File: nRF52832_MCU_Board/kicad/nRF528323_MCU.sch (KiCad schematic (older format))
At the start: 34 parts, among them J6 DEBUG_CONNECTOR, J7 CONN_01X05, J8 MM8130-2600, X1 32MHz, X2 32.768kHz

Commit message: Update KiCad Project nRF52832_MCU_Board
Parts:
- J6: footprint Nordic_misc:Pin_Header_Straight_2x05_Pitch1.27mm_SMD -> Nordic_misc:ftsh-105-01-l-dv
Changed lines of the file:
@@
 F 0 "J6" H 7500 5200 50  0000 C CNN
 F 1 "DEBUG_CONNECTOR" H 7500 4600 50  0000 C CNN
-F 2 "Nordic_misc:Pin_Header_Straight_2x05_Pitch1.27mm_SMD" H 7500 3700 50  0001 C CNN
+F 2 "Nordic_misc:ftsh-105-01-l-dv" H 7500 3700 50  0001 C CNN
 F 3 "" H 7500 3700 50  0001 C CNN
 	1    7500 4900

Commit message: Update KiCAD Project nRF52832_MCU_Board
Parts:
- X1: footprint Crystals:Crystal_SMD_2016-4pin_2.0x1.6mm -> Nordic_nRF:Crystal_SMD_2016-4pin_2.0x1.6mm
- X2: footprint Crystals:Crystal_SMD_3215-2pin_3.2x1.5mm -> Nordic_nRF:Crystal_SMD_3215-2pin_3.2x1.5mm
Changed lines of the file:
@@
 $Descr USLetter 11000 8500
 encoding utf-8
-Sheet 2 4
+Sheet 4 4
 Title ""
 Date "2017-07-22"
@@
 F 0 "X2" V 2000 2950 50  0000 C CNN
 F 1 "32.768kHz" V 2150 3050 50  0000 C CNN
-F 2 "Crystals:Crystal_SMD_3215-2pin_3.2x1.5mm" H 2050 2800 50  0001 C CNN
+F 2 "Nordic_nRF:Crystal_SMD_3215-2pin_3.2x1.5mm" H 2050 2800 50  0001 C CNN
 F 3 "" H 2050 2800 50  0001 C CNN
 	1    2050 2800
@@
 F 0 "X1" V 8450 2500 50  0000 L CNN
 F 1 "32MHz" V 8550 2300 50  0000 L CNN
-F 2 "Crystals:Crystal_SMD_2016-4pin_2.0x1.6mm" H 8650 2700 50  0001 C CNN
+F 2 "Nordic_nRF:Crystal_SMD_2016-4pin_2.0x1.6mm" H 8650 2700 50  0001 C CNN
 F 3 "" H 8650 2700 50  0001 C CNN
 	1    8650 2700

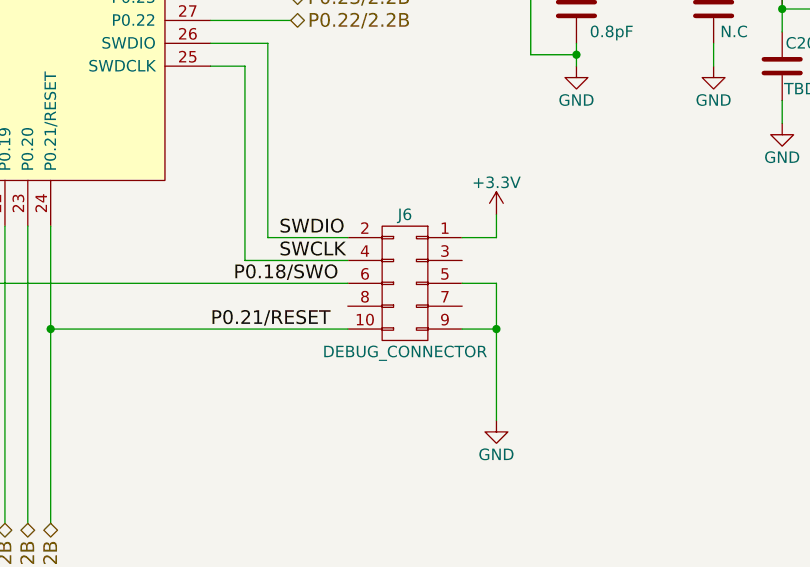
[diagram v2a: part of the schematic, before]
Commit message: Update KiCAD Project nRF52832_MCU_Board
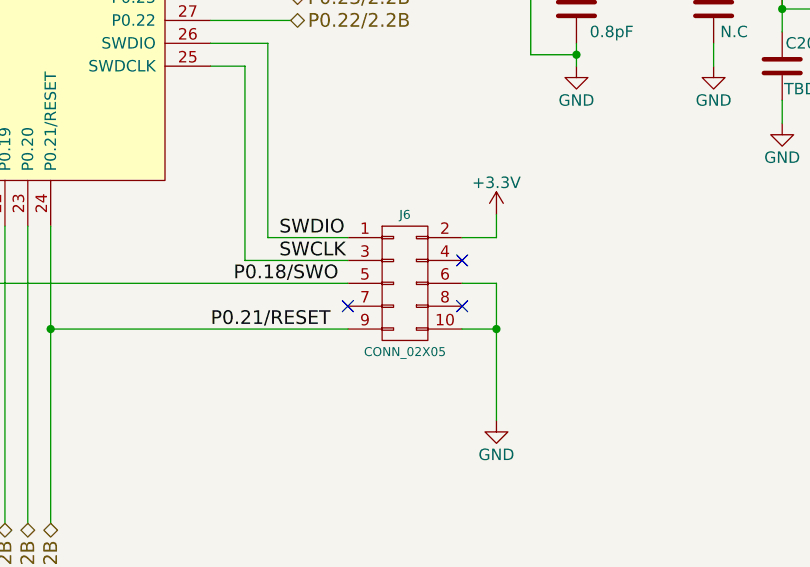
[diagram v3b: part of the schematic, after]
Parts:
- J6: value DEBUG_CONNECTOR -> CONN_02X05
- nRF1: footprint nRF52:UQFN-48-1EP_6x6mm_Pitch0.4mm -> Nordic_nRF:Nordic_nRF-QFN40P600X600X90-48_N
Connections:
- net +3V3: now also J6.2 (P2); no longer J6.1 (P1)
- net GND: now also J6.10 (P10), J6.6 (P6); no longer J6.5 (P5), J6.9 (P9)
- net P0.18/SWO/2.2B: now also J6.5 (P5); no longer J6.6 (P6)
- net P0.21/RESET/2.2B: now also J6.9 (P9); no longer J6.10 (P10)
- net SWCLK: now also J6.3 (P3); no longer J6.4 (P4)
- net SWDIO: now also J6.1 (P1); no longer J6.2 (P2)
- no-connect marks 3 -> 6
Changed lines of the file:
@@
 EESchema Schematic File Version 2
-LIBS:power
-LIBS:device
-LIBS:transistors
-LIBS:conn
-LIBS:linear
-LIBS:regul
+LIBS:nRF52832_MCU_Board-rescue
+LIBS:Nordic_misc
+LIBS:Nordic_nRF
+LIBS:74xgxx
 LIBS:74xx
-LIBS:cmos4000
-LIBS:adc-dac
-LIBS:memory
-LIBS:xilinx
-LIBS:microcontrollers
-LIBS:dsp
-LIBS:microchip
-LIBS:analog_switches
-LIBS:motorola
-LIBS:texas
-LIBS:intel
-LIBS:audio
-LIBS:interface
-LIBS:digital-audio
-LIBS:philips
-LIBS:display
-LIBS:cypress
-LIBS:siliconi
-LIBS:opto
-LIBS:atmel
-LIBS:contrib
-LIBS:valves
-LIBS:74xgxx
 LIBS:ac-dc
 LIBS:actel
+LIBS:adc-dac
 LIBS:allegro
 LIBS:Altera
 LIBS:analog_devices
+LIBS:analog_switches
+LIBS:atmel
+LIBS:audio
 LIBS:battery_management
 LIBS:bbd
@@
 LIBS:brooktre
 LIBS:cmos_ieee
+LIBS:cmos4000
+LIBS:conn
+LIBS:contrib
+LIBS:cypress
 LIBS:dc-dc
+LIBS:device
+LIBS:digital-audio
 LIBS:diode
+LIBS:display
+LIBS:dsp
 LIBS:elec-unifil
 LIBS:ESD_Protection
@@
 LIBS:graphic
 LIBS:hc11
+LIBS:intel
+LIBS:interface
 LIBS:ir
 LIBS:Lattice
 LIBS:leds
+LIBS:linear
 LIBS:logo
 LIBS:maxim
 LIBS:mechanical
+LIBS:memory
+LIBS:microchip
 LIBS:microchip_dspic33dsc
 LIBS:microchip_pic10mcu
@@
 LIBS:microchip_pic24mcu
 LIBS:microchip_pic32mcu
+LIBS:microcontrollers
 LIBS:modules
 LIBS:motor_drivers
+LIBS:motorola
 LIBS:motors
 LIBS:msp430
@@
 LIBS:nxp_armmcu
 LIBS:onsemi
-LIBS:OPA4134
+LIBS:opto
 LIBS:Oscillators
-LIBS:PCM3168A
+LIBS:philips
+LIBS:power
+LIBS:Power_Management
 LIBS:powerint
-LIBS:Power_Management
 LIBS:pspice
 LIBS:references
+LIBS:regul
 LIBS:relays
 LIBS:rfcom
 LIBS:sensors
 LIBS:silabs
+LIBS:siliconi
 LIBS:stm8
 LIBS:stm32
 LIBS:supertex
 LIBS:switches
-LIBS:TMS320VC5502
+LIBS:texas
 LIBS:transf
+LIBS:transistors
 LIBS:triac_thyristor
-LIBS:TS3A27518E
 LIBS:ttl_ieee
+LIBS:valves
 LIBS:video
 LIBS:w_analog
-LIBS:w_connectors
 LIBS:w_device
-LIBS:wiznet
 LIBS:w_logic
 LIBS:w_memory
 LIBS:w_microcontrollers
 LIBS:w_opto
-LIBS:Worldsemi
 LIBS:w_relay
 LIBS:w_rtx
 LIBS:w_transistor
 LIBS:w_vacuum
+LIBS:wiznet
+LIBS:Worldsemi
 LIBS:Xicor
+LIBS:xilinx
 LIBS:zetex
 LIBS:Zilog
-LIBS:Nordic_misc
-LIBS:Nordic_nRF
 LIBS:nRF52832_MCU_Board-cache
 EELAYER 25 0
@@
 F 0 "nRF1" H 5400 3600 60  0000 C CNN
 F 1 "nRF52832" H 5400 3400 60  0000 C CNN
-F 2 "nRF52:UQFN-48-1EP_6x6mm_Pitch0.4mm" H 5400 3400 60  0001 C CNN
+F 2 "Nordic_nRF:Nordic_nRF-QFN40P600X600X90-48_N" H 5400 3400 60  0001 C CNN
 F 3 "" H 5400 3400 60  0001 C CNN
 	1    5400 3400
@@
 Wire Wire Line
 	6900 3850 6900 4700
-$Comp
-L CONN_02X05 J6
-U 1 1 597D61D5
-P 7500 4900
-F 0 "J6" H 7500 5200 50  0000 C CNN
-F 1 "DEBUG_CONNECTOR" H 7500 4600 50  0000 C CNN
-F 2 "Nordic_misc:ftsh-105-01-l-dv" H 7500 3700 50  0001 C CNN
-F 3 "" H 7500 3700 50  0001 C CNN
-	1    7500 4900
-	-1   0    0    -1
-$EndComp
 Wire Wire Line
 	6900 4700 7250 4700
@@
 U 1 1 597D20DE
 P 9150 3450
+AR Path="/597D20DE" Ref="J8"  Part="1"
+AR Path="/597D109B/597D20DE" Ref="J8"  Part="1"
 F 0 "J8" H 9160 3570 50  0000 C CNN
 F 1 "MM8130-2600" H 9500 3450 50  0000 C CNN
@@
 	9900 3700 9150 3700
 Connection ~ 9150 3700
+$Comp
+L CONN_02X05 J6
+U 1 1 597F8B91
+P 7500 4900
+F 0 "J6" H 7500 5200 39  0000 C CNN
+F 1 "CONN_02X05" H 7500 4600 39  0000 C CNN
+F 2 "Nordic_misc:ftsh-105-01-l-dv" H 7500 3700 50  0001 C CNN
+F 3 "" H 7500 3700 50  0001 C CNN
+	1    7500 4900
+	1    0    0    -1
+$EndComp
+NoConn ~ 7750 4800
+NoConn ~ 7750 5000
+NoConn ~ 7250 5000
 $EndSCHEMATC
